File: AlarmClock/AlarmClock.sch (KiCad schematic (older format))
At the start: 39 parts, among them Q1 2N3904, Q2 2N3904, Q3 2N3904, Q4 2N3904, Q5 2N3904, SW1 SW_Push_Dual, SW2 SW_Push_Dual, SW3 SW_Push_Dual, SW4 SW_Push_Dual, SW5 SW_Push_Dual, U1 LM386, U2 LTC-4727JR, U3 LM358

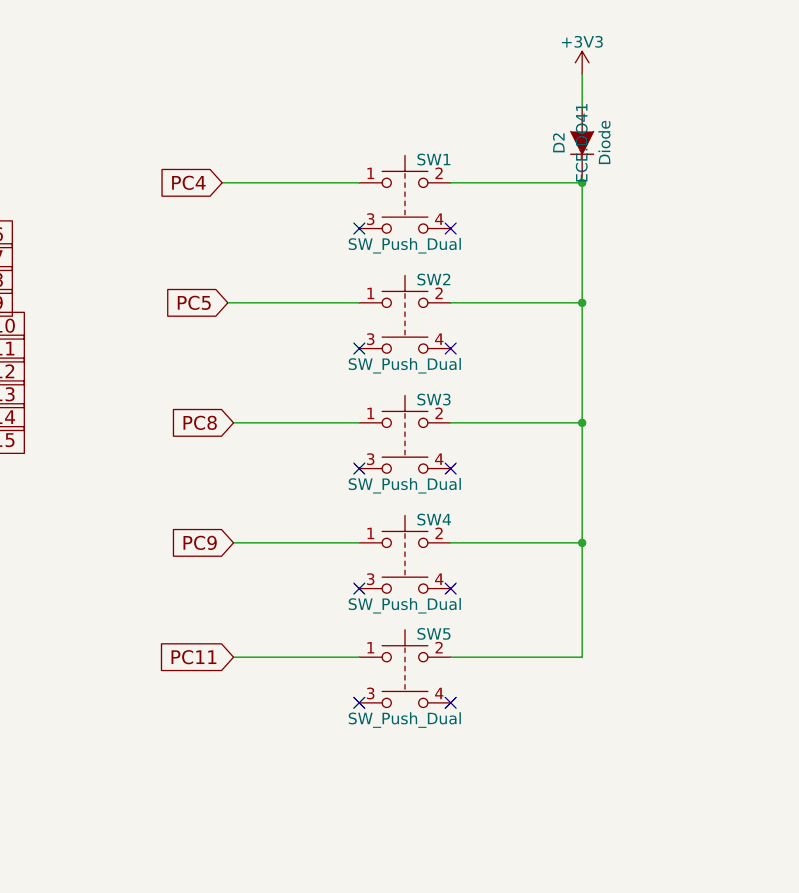
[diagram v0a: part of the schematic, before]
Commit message: geber files and final pcb
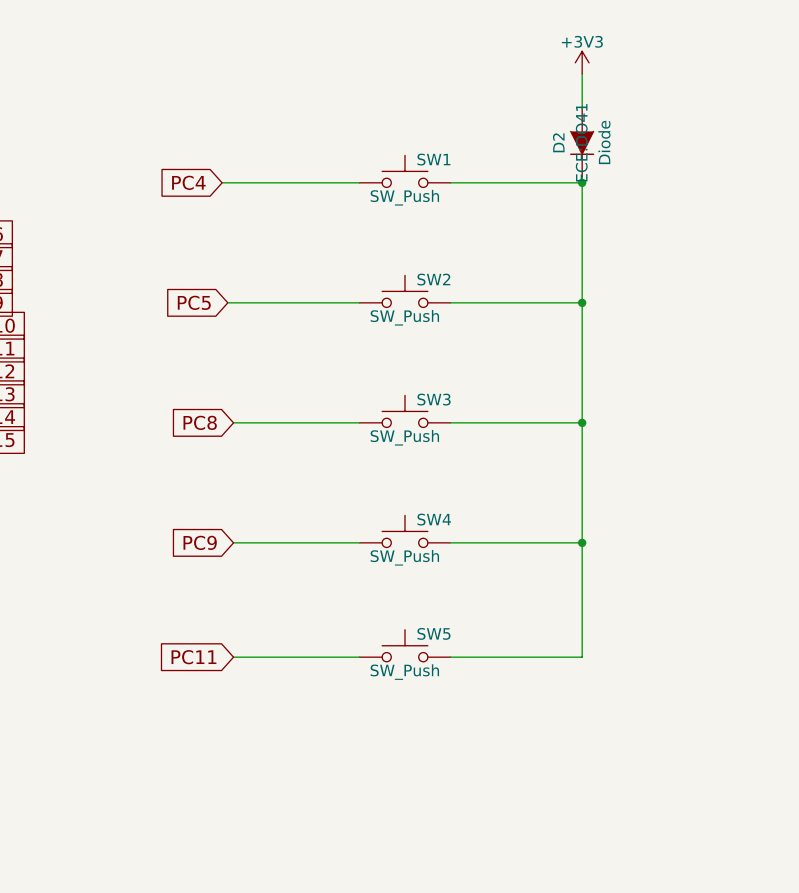
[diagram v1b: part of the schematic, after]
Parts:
- removed SW1, SW2, SW3, SW4, SW5: SW_Push_Dual, Buttons_Switches_THT:SW_PUSH_6mm, symbol SW_Push_Dual
- added SW1, SW2, SW3, SW4, SW5: SW_Push, Buttons_Switches_THT:SW_PUSH_6mm, symbol SW_Push
- LS1: footprint Wire_Pads:SolderWirePad_2x_1mmDrill -> Wire_Connections_Bridges:WireConnection_1.00mmDrill
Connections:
- net PC11: now also SW5.1
- net PC4: now also SW1.1
- net PC5: now also SW2.1
- net PC8: now also SW3.1
- net PC9: now also SW4.1
- net at D2.K (Cathode): now also SW1.2, SW2.2, SW3.2, SW4.2, SW5.2
- no-connect marks 80 -> 70
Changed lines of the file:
@@
 F 0 "LS1" H 3950 2475 50  0000 R CNN
 F 1 "Speaker" H 3950 2400 50  0000 R CNN
-F 2 "Wire_Pads:SolderWirePad_2x_1mmDrill" H 3900 2050 50  0001 C CNN
+F 2 "Wire_Connections_Bridges:WireConnection_1.00mmDrill" H 3900 2050 50  0001 C CNN
 F 3 "" H 3890 2200 50  0001 C CNN
 	1    3900 2250
@@
 $EndComp
 $Comp
-L SW_Push_Dual SW1
-U 1 1 5B3BDA0C
-P 9275 3475
-F 0 "SW1" H 9325 3575 50  0000 L CNN
-F 1 "SW_Push_Dual" H 9275 3205 50  0000 C CNN
-F 2 "Buttons_Switches_THT:SW_PUSH_6mm" H 9275 3675 50  0001 C CNN
-F 3 "" H 9275 3675 50  0001 C CNN
-	1    9275 3475
-	1    0    0    -1
-$EndComp
-$Comp
-L SW_Push_Dual SW2
-U 1 1 5B3BDD20
-P 9275 4000
-F 0 "SW2" H 9325 4100 50  0000 L CNN
-F 1 "SW_Push_Dual" H 9275 3730 50  0000 C CNN
-F 2 "Buttons_Switches_THT:SW_PUSH_6mm" H 9275 4200 50  0001 C CNN
-F 3 "" H 9275 4200 50  0001 C CNN
-	1    9275 4000
-	1    0    0    -1
-$EndComp
-$Comp
-L SW_Push_Dual SW3
-U 1 1 5B3BDD87
-P 9275 4525
-F 0 "SW3" H 9325 4625 50  0000 L CNN
-F 1 "SW_Push_Dual" H 9275 4255 50  0000 C CNN
-F 2 "Buttons_Switches_THT:SW_PUSH_6mm" H 9275 4725 50  0001 C CNN
-F 3 "" H 9275 4725 50  0001 C CNN
-	1    9275 4525
-	1    0    0    -1
-$EndComp
-$Comp
-L SW_Push_Dual SW4
-U 1 1 5B3BDEC7
-P 9275 5050
-F 0 "SW4" H 9325 5150 50  0000 L CNN
-F 1 "SW_Push_Dual" H 9275 4780 50  0000 C CNN
-F 2 "Buttons_Switches_THT:SW_PUSH_6mm" H 9275 5250 50  0001 C CNN
-F 3 "" H 9275 5250 50  0001 C CNN
-	1    9275 5050
-	1    0    0    -1
-$EndComp
-$Comp
-L SW_Push_Dual SW5
-U 1 1 5B3BE993
-P 9275 5550
-F 0 "SW5" H 9325 5650 50  0000 L CNN
-F 1 "SW_Push_Dual" H 9275 5280 50  0000 C CNN
-F 2 "Buttons_Switches_THT:SW_PUSH_6mm" H 9275 5750 50  0001 C CNN
-F 3 "" H 9275 5750 50  0001 C CNN
-	1    9275 5550
-	1    0    0    -1
-$EndComp
-$Comp
 L +3V3 #PWR015
 U 1 1 5B3BF19D
@@
 Wire Wire Line
 	9075 3475 8475 3475
-NoConn ~ 9075 3675
-NoConn ~ 9475 3675
-NoConn ~ 9075 4200
-NoConn ~ 9475 4200
-NoConn ~ 9075 4725
-NoConn ~ 9475 4725
-NoConn ~ 9075 5250
-NoConn ~ 9475 5250
-NoConn ~ 9075 5750
-NoConn ~ 9475 5750
 $Comp
 L Diode D1
@@
 Connection ~ 10350 1700
 Connection ~ 1850 1350
+$Comp
+L SW_Push SW1
+U 1 1 5B3C2F2D
+P 9275 3475
+F 0 "SW1" H 9325 3575 50  0000 L CNN
+F 1 "SW_Push" H 9275 3415 50  0000 C CNN
+F 2 "Buttons_Switches_THT:SW_PUSH_6mm" H 9275 3675 50  0001 C CNN
+F 3 "" H 9275 3675 50  0001 C CNN
+	1    9275 3475
+	1    0    0    -1
+$EndComp
+$Comp
+L SW_Push SW2
+U 1 1 5B3C2FB8
+P 9275 4000
+F 0 "SW2" H 9325 4100 50  0000 L CNN
+F 1 "SW_Push" H 9275 3940 50  0000 C CNN
+F 2 "Buttons_Switches_THT:SW_PUSH_6mm" H 9275 4200 50  0001 C CNN
+F 3 "" H 9275 4200 50  0001 C CNN
+	1    9275 4000
+	1    0    0    -1
+$EndComp
+$Comp
+L SW_Push SW3
+U 1 1 5B3C301B
+P 9275 4525
+F 0 "SW3" H 9325 4625 50  0000 L CNN
+F 1 "SW_Push" H 9275 4465 50  0000 C CNN
+F 2 "Buttons_Switches_THT:SW_PUSH_6mm" H 9275 4725 50  0001 C CNN
+F 3 "" H 9275 4725 50  0001 C CNN
+	1    9275 4525
+	1    0    0    -1
+$EndComp
+$Comp
+L SW_Push SW4
+U 1 1 5B3C30A4
+P 9275 5050
+F 0 "SW4" H 9325 5150 50  0000 L CNN
+F 1 "SW_Push" H 9275 4990 50  0000 C CNN
+F 2 "Buttons_Switches_THT:SW_PUSH_6mm" H 9275 5250 50  0001 C CNN
+F 3 "" H 9275 5250 50  0001 C CNN
+	1    9275 5050
+	1    0    0    -1
+$EndComp
+$Comp
+L SW_Push SW5
+U 1 1 5B3C3113
+P 9275 5550
+F 0 "SW5" H 9325 5650 50  0000 L CNN
+F 1 "SW_Push" H 9275 5490 50  0000 C CNN
+F 2 "Buttons_Switches_THT:SW_PUSH_6mm" H 9275 5750 50  0001 C CNN
+F 3 "" H 9275 5750 50  0001 C CNN
+	1    9275 5550
+	1    0    0    -1
+$EndComp
 $EndSCHEMATC
